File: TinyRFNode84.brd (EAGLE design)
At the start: 32 x 42.6 mm, 14 parts, among them IC3 MCP1703CB, T1 2N2222, U1 ATTINY84-20SSU

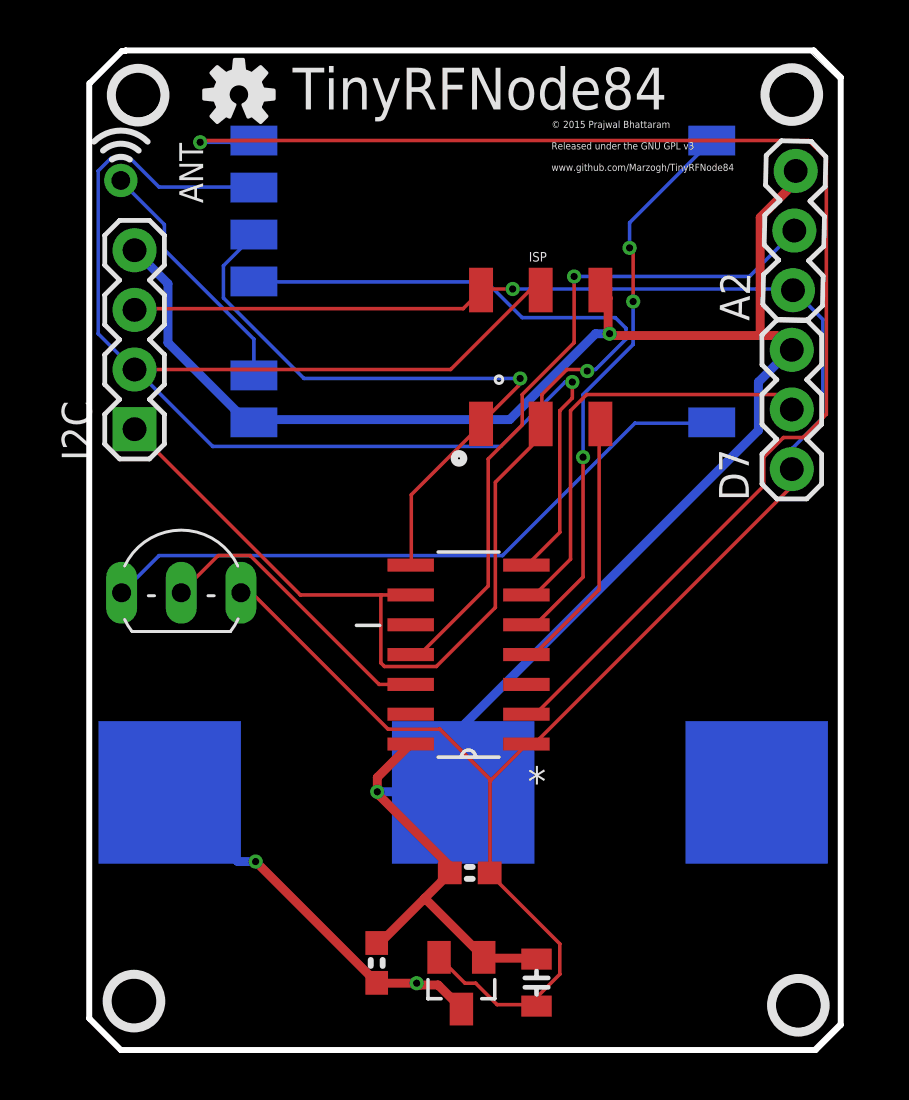
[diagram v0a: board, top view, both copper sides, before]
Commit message: v2.0.2
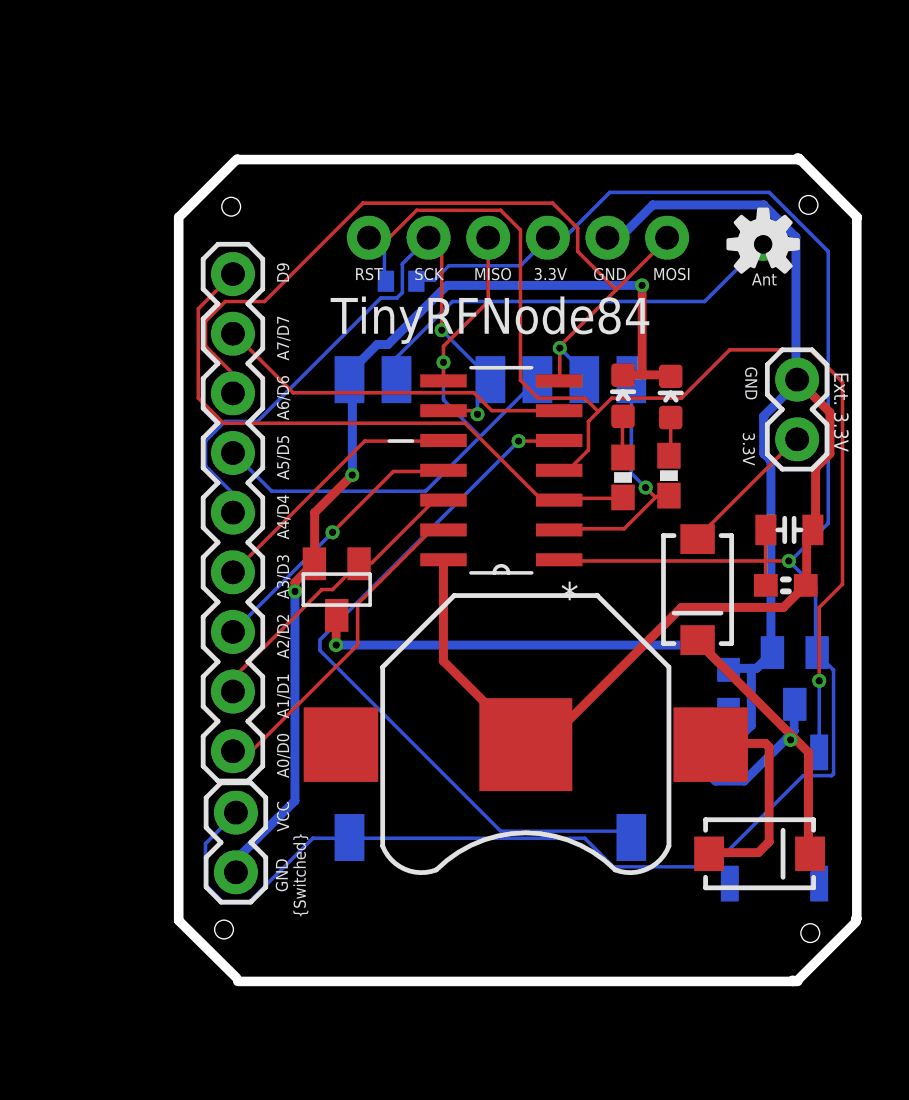
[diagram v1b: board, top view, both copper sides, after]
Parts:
- removed A2, D7: (no value), SparkFun-Connectors:1X03
- removed I2C: (no value), SparkFun-Connectors:1X04
- removed ISP: (no value), SparkFun-Connectors:2X3_SMD
- removed T1: 2N2222, adafruit:TO92-EBC-OVAL
- added D1: RED, SparkFun-LED:LED-0603
- added D2: GREEN, SparkFun-LED:LED-0603
- added D3, D4: MBRA140, SparkFun-DiscreteSemi:SMA-DIODE
- added ICSP: ICSP, SparkFun-Connectors:1X06_NO_SILK
- added JP1: M09, SparkFun-Connectors:1X09
- added JP2, JP3: M02PTH, SparkFun-Connectors:1X02
- added Q1: MOSFET-NCHANNELBSS138, SparkFun-DiscreteSemi:SOT23
- added R1, R2: 220, SparkFun-Passives:0603-RES
- added R3: 4k7, SparkFun-Passives:0402-RES
- added S1: RESET, SparkFun-Electromechanical:TACTILE-SWITCH-SMD
- added U$3: (no value), SparkFun-Aesthetics:OSHW-LOGO-S
- BAT1: device SparkFun-Electromechanical:BATTCON_20MM -> SparkFun-Electromechanical:BATTCON_12MM
- moved U$1 27.5 mm to (29.1, 34.3)
- moved U$2 23.2 mm to (29.1, 34.3), flipped to the bottom
- moved C3 22.1 mm to (30.2, 22.1), turned to 0 degrees
- moved IC3 19.2 mm to (30.4, 15.8), flipped to the bottom
- moved C2 19.0 mm to (27.6, 15.3), flipped to the bottom
- moved C4 18.2 mm to (30.0, 19.8), turned to 0 degrees
- moved U$5 13.5 mm to (18.5, 20.5), turned to 90 degrees
- moved U1 7.97 mm to (17.9, 24.7)
- moved BAT1 3.35 mm to (19.0, 13.0), flipped to the top
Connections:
- net D8 renamed D8/INT0
- removed net AREF: U1.13
- removed net D1: T1.B, U1.12
- removed net D2: A2.2, U1.11
- removed net D3: U1.10
- removed net D7: D7.2, U1.6
- removed net SS: U$5.NSS, U1.2
- removed net VDD: T1.E, U$5.VDD
- new net 3V: C2.1, D3.C, D4.C, IC3.3
- new net BAT: BAT1.PWR@1, D3.A
- new net D0/A0/AREF: JP1.9, U1.13
- new net D1/A1: JP1.8, Q1.1, U1.12
- new net D10/SS: R1.2, U$5.NSS, U1.2
- new net D2/A2: JP1.7, U1.11
- new net D3/A3: JP1.6, U1.10
- new net D7/A7: JP1.2, U1.6
- new net N$12: D1.A, R2.1
- new net N$13: D2.A, R1.1
- new net SW_GND: D1.C, D2.C, JP3.1, Q1.2, U$5.GND
- net D9: now also JP1.1, R2.2
- net GND: now also BAT1.GND, ICSP.5, JP2.1, Q1.3, S1.1; no longer A2.3, BAT1.2, D7.3, I2C.4, ISP.6, U$5.GND
- net MISO: now also ICSP.3, JP1.4; no longer ISP.1
- net MOSI/SDA: now also ICSP.6, JP1.3; no longer I2C.2, ISP.4
- net PWR: now also D4.A, JP2.2; no longer BAT1.1, C2.1, IC3.3
- net RST: now also ICSP.1, R3.1, S1.3; no longer ISP.5
- net SCK/SCL: now also ICSP.2, JP1.5; no longer I2C.1, ISP.3
- net VCC: now also ICSP.4, JP3.2, R3.2, U$5.VDD; no longer A2.1, D7.1, I2C.3, ISP.2, T1.C
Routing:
- net SS: track 59.1 -> 0.00 mm, vias 1 -> 0
- net SW_GND: track 0.00 -> 43.3 mm, vias 0 -> 3
- net RST: track 11.3 -> 51.4 mm, vias 0 -> 1
- net MOSI/SDA: track 64.9 -> 35.0 mm
- net D2: track 29.4 -> 0.00 mm, vias 1 -> 0
- net VDD: track 28.1 -> 0.00 mm
- net SCK/SCL: track 55.2 -> 27.7 mm, vias 1 -> 2
- net D9: track 0.00 -> 25.8 mm
- net 3V: track 0.00 -> 20.2 mm, vias 0 -> 1
- net D7: track 18.8 -> 0.00 mm
- net D7/A7: track 0.00 -> 15.3 mm
- net D0/A0/AREF: track 0.00 -> 13.9 mm
- net D1/A1: track 0.00 -> 12.7 mm
- net D1: track 12.7 -> 0.00 mm
- net D2/A2: track 0.00 -> 11.8 mm, vias 0 -> 1
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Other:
- board size 32 x 42.6 mm -> 28.9 x 35.1 mm
- board text added: "3.3V"
- board text added: "A0/D0"
- board text added: "A1/D1"
- board text added: "A2/D2"
- board text added: "A3/D3"
- board text added: "A4/D4"
- board text added: "A5/D5"
- board text added: "A6/D6"
- board text added: "A7/D7"
- board text added: "Ant"
- board text added: "D9"
- board text added: "Ext. 3.3V"
- board text added: "GND"
- board text added: "GND {Switched}"
- board text added: "MISO"
- board text added: "MOSI"
- board text added: "RST"
- board text added: "SCK"
- board text added: "VCC"
- board text added: "© GNU GPL v3 2015 Prajwal Bhattaram www.github.com/Marzogh/TinyRFNode84"
- board text removed: "ANT"
- board text removed: "© 2015 Prajwal Bhattaram Released under the GNU GPL v3 www.github.com/Marzogh/TinyRFNode84"
